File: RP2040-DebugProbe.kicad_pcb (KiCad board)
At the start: 2 copper layers, 59.7 x 25.4 mm, 60 parts, among them J1 CONN_MCU_JTAG, J10 CONN_USB, J2 CONN_MCU_UART, J3 CONN_DBG_COMB, J4 CONN_3V3_JUMPER, J7 CONN_DBG_JTAG, SW1 BOOTSEL, U1 W25Q128JVS, U2 RP2040, U3 74AUP1T17, U4 W25Q128JVEIQ, U5 AMS1117-3.3, U6 74AUP1T17, Y1 12MHz

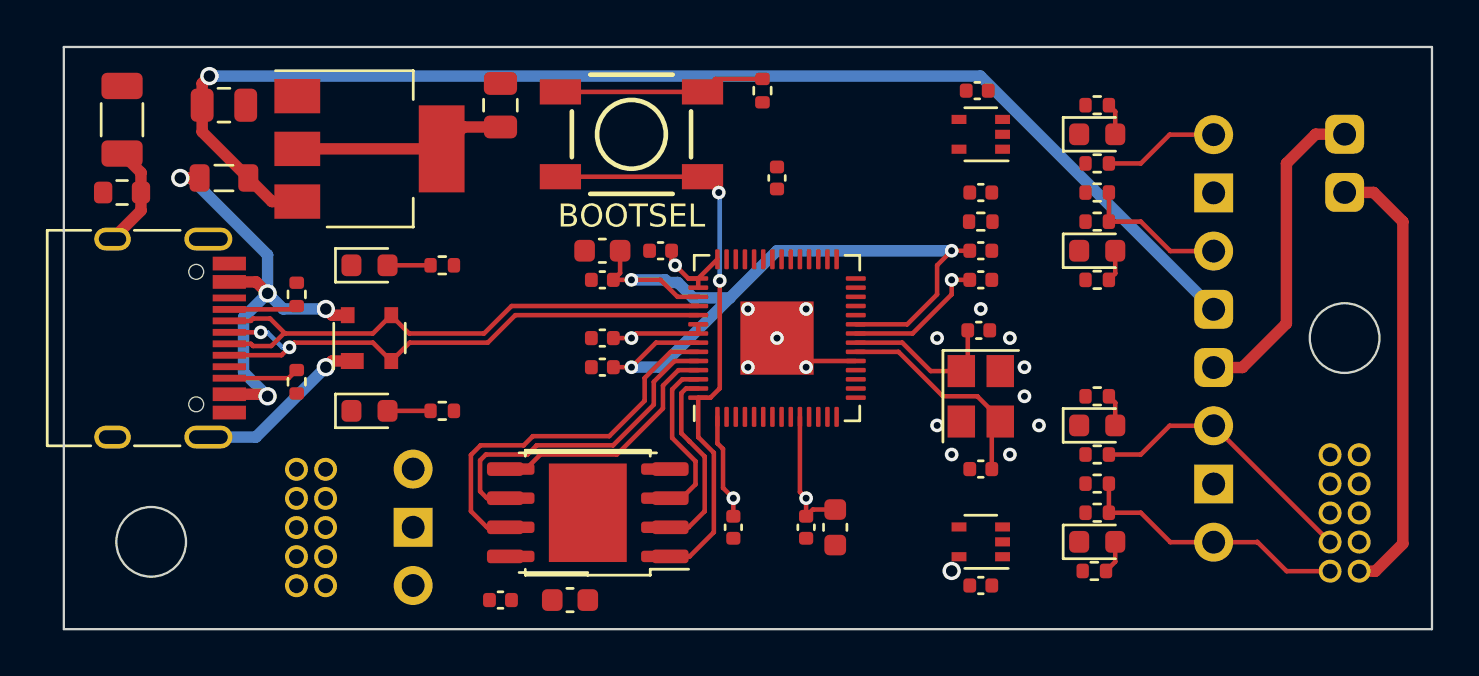
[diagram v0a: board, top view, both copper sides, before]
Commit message: Moved stuff around
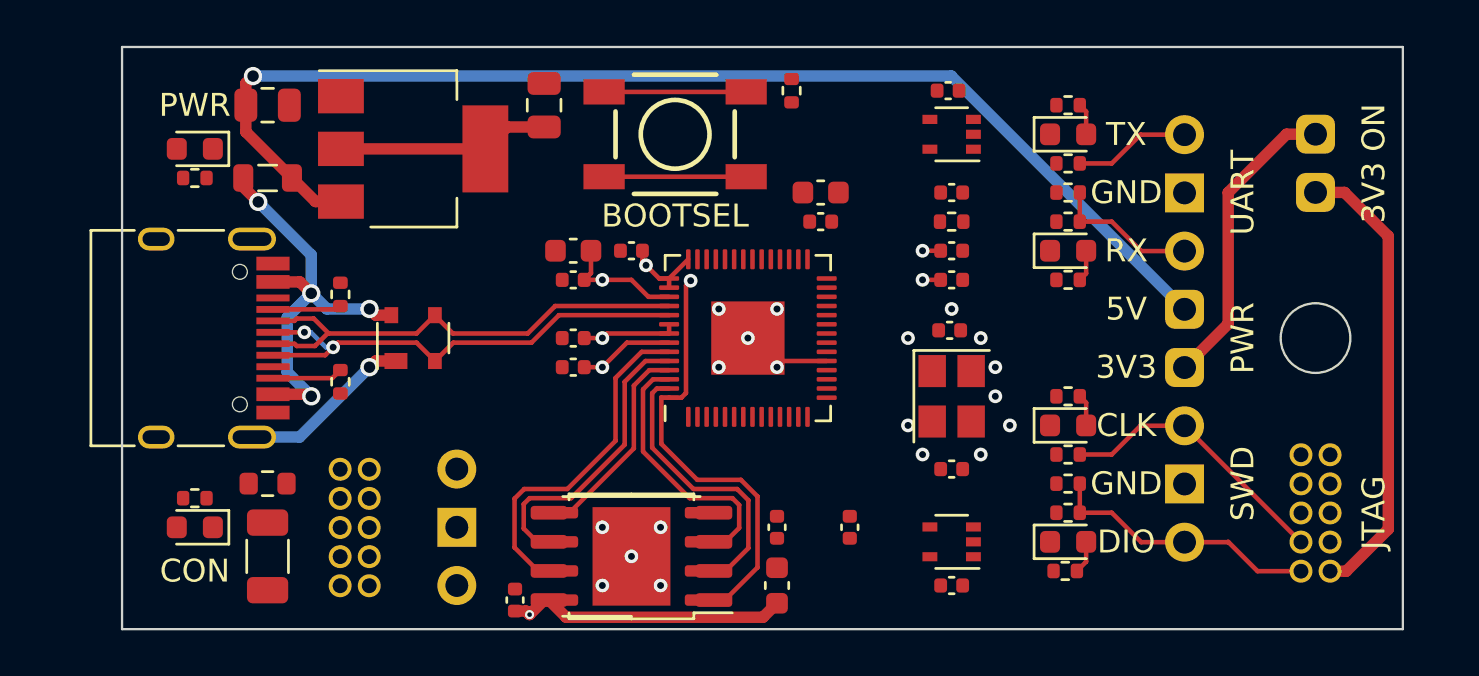
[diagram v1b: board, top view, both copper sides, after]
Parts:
- moved C21 20.1 mm to (133.3, 117.5), turned to -90 degrees
- moved C1 14.6 mm to (157.5, 101.6), turned to 0 degrees
- moved R12 14.2 mm to (133.3, 114.3), turned to 0 degrees
- moved R3 11.4 mm to (130.2, 114.9)
- moved R6 11.4 mm to (130.2, 101.0)
- moved D2 9.16 mm to (130.2, 99.7), turned to 180 degrees
- moved D5 9.16 mm to (130.2, 116.2), turned to 180 degrees
- moved C16 9.05 mm to (155.6, 118.7), turned to 90 degrees
- moved C4 2.69 mm to (157.5, 102.9), turned to 0 degrees
- moved U1 2.69 mm to (149.2, 117.5)
- moved U4 2.69 mm to (149.2, 117.5)
- moved C10 1.91 mm to (158.8, 116.2)
- moved C14 1.91 mm to (145.4, 97.8)
- moved C15 1.91 mm to (133.3, 97.8)
- moved C3 1.91 mm to (155.6, 116.2)
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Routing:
- net +1V1: track 37.3 -> 10.3 mm
- net XIN: track 9.85 -> 0.00 mm
- net XOUT: track 7.01 -> 0.00 mm
- net SHIELD: track 12.2 -> 7.66 mm
- net +3V3: track 48.5 -> 44.1 mm, vias 6 -> 4
- net QSPI_SD2: track 7.23 -> 11.5 mm
- net QSPI_SD1: track 8.22 -> 12.3 mm
- net USB_DP: track 24.7 -> 21.6 mm
- net USB_DN: track 24.6 -> 21.5 mm
- net VUSB: track 56.0 -> 52.8 mm
- net Net-(R7-Pad1): track 9.05 -> 6.20 mm
- net Net-(D5-A): track 1.88 -> 0.00 mm
- net Net-(D2-A): track 1.88 -> 0.00 mm
- net QSPI_SD3: track 16.6 -> 15.1 mm
- net QSPI_SCLK: track 14.5 -> 12.9 mm
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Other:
- board size 59.7 x 25.4 mm -> 55.9 x 25.4 mm
- board text added: "3V3"
- board text added: "3V3 ON"
- board text added: "5V"
- board text added: "CLK"
- board text added: "CON"
- board text added: "DIO"
- board text added: "GND"
- board text added: "JTAG"
- board text added: "PWR"
- board text added: "RX"
- board text added: "SWD"
- board text added: "TX"
- board text added: "UART"
